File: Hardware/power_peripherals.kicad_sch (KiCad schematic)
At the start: 46 parts, among them J10 microSD_Friction, J11 Qwiic_RA, J5 Conn_01x10, J6 Conn_01x10, J7 Conn_01x10, J8 Conn_01x10, J9 JST_2mm_LiPo, Q1 DMG2305UX, SW2 SMD_4.6x2.8mm_h2.5mm, SW3 SMD_4.6x2.8mm_h2.5mm, SW4 SMD_4.6x2.8mm_h2.5mm, U6 LM66200, U7 RT9080-3.3, U8 MCP73831, U9 MAX17048

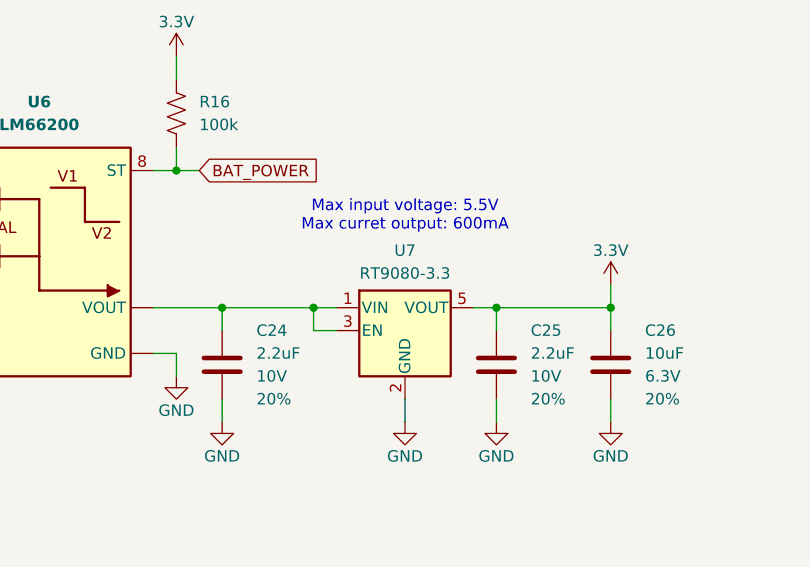
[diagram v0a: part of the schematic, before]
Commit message: Library update
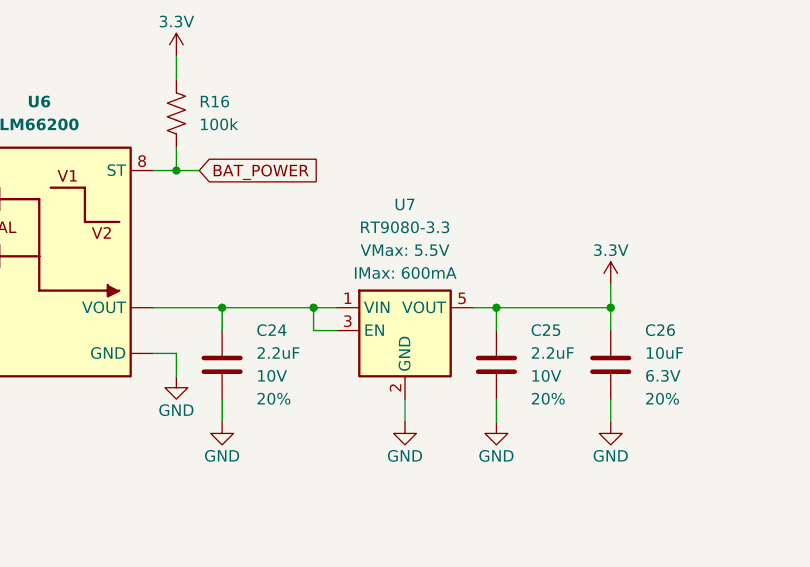
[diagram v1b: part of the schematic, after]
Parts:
- D5: footprint SparkFun-LED:LED_0603_1608Metric -> SparkFun-LED:LED_0603_1608Metric_Red
- D6: footprint SparkFun-LED:LED_0603_1608Metric -> SparkFun-LED:LED_0603_1608Metric_Yellow
- U7: IMax (none) -> 600mA; VMax 6V -> 5.5V
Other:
- note removed: "Max input voltage: 5.5V Max curret output: 600mA"
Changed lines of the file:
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@@
 		)
 	)
-	(text "Max input voltage: 5.5V\nMax curret output: 600mA"
-		(exclude_from_sim no)
-		(at 91.44 53.34 0)
-		(effects
-			(font
-				(size 1.27 1.27)
-			)
-		)
-	)
 	(global_label "XBLR_IO2"
 		(shape input)
@@
 			)
 		)
-		(property "Footprint" "SparkFun-LED:LED_0603_1608Metric"
+		(property "Footprint" "SparkFun-LED:LED_0603_1608Metric_Red"
 			(at 217.17 229.87 0)
 			(effects
@@
 			)
 		)
-		(property "Footprint" "SparkFun-LED:LED_0603_1608Metric"
+		(property "Footprint" "SparkFun-LED:LED_0603_1608Metric_Yellow"
 			(at 211.074 69.85 0)
 			(effects
@@
 		(fields_autoplaced yes)
 		(property "Reference" "U7"
-			(at 91.44 57.15 0)
+			(at 91.44 52.07 0)
 			(effects
 				(font
@@
 		)
 		(property "Value" "RT9080-3.3"
-			(at 91.44 59.69 0)
+			(at 91.44 54.61 0)
 			(effects
 				(font
@@
 			)
 		)
-		(property "VMax" "6V"
-			(at 91.44 85.09 0)
+		(property "VMax" "5.5V"
+			(at 91.44 57.15 0)
+			(show_name yes)
 			(effects
 				(font
 					(size 1.27 1.27)
 				)
-				(hide yes)
 			)
 		)
@@
 			)
 		)
+		(property "IMax" "600mA"
+			(at 91.44 59.69 0)
+			(show_name yes)
+			(effects
+				(font
+					(size 1.27 1.27)
+				)
+			)
+		)
